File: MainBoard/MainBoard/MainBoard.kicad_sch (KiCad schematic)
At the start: 40 parts, among them IC1 BQ25171QWDRCRQ1, J1 KH-TYPE-C-16P, U1 STM32L496VGY6PTR, U2 MX25R1635FZUIL0, U3 SI3477DV-T1-GE3, U4 SI3477DV-T1-GE3, U5 TPS63802DLAR, U6 FUSB302BMPX

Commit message: Schematic work
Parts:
- added C21: 1uF, Capacitor_SMD:C_0402_1005Metric_Pad0.74x0.62mm_HandSolder, symbol Device:C
- added C22: 100nF, Capacitor_SMD:C_0402_1005Metric_Pad0.74x0.62mm_HandSolder, symbol Device:C
- added C23, C24: 470pF, Capacitor_SMD:C_0402_1005Metric_Pad0.74x0.62mm_HandSolder, symbol Device:C
- added R8, R9: 4.7k, Resistor_SMD:R_0402_1005Metric_Pad0.72x0.64mm_HandSolder, symbol Device:R_US
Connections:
- net +3.3V: now also C19.1, C20.1, R6.1, U5.6 (VOUT), U6.3 (VDD), U6.4 (VDD), C21.1, C22.1
- net GND: now also U6.15 (EPAD), U6.8 (GND), U6.9 (GND), C21.2, C22.2, C23.2, C24.2, R8.2, R9.1
- net at D1.2 (A), J1.A4_B9 (VBUS), J1.A9_B4 (VBUS): now also U6.2 (VBUS)
- net at J1.A5 (CC1): now also U6.11 (CC1), C24.1
- net at J1.B5 (CC2): now also U6.14 (CC2), C23.1
- net I2C1_SCL: now reaches U6.6 (SCL)
- net I2C1_SCL: now also R8.1
- net I2C1_SDA: now reaches U6.7 (SDA)
- net I2C1_SDA: now also R9.2
- no-connect marks 9 -> 12
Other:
- note added: "3.3V Regulator"
- note added: "Batteries"
- note added: "Battery Managment"
- note added: "Extra Flash"
- note added: "USBC + PD"
- moved on the sheet: BT1, BT2, C1, C10, C11, C12, C13, C14, C15, C16, C17, C18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

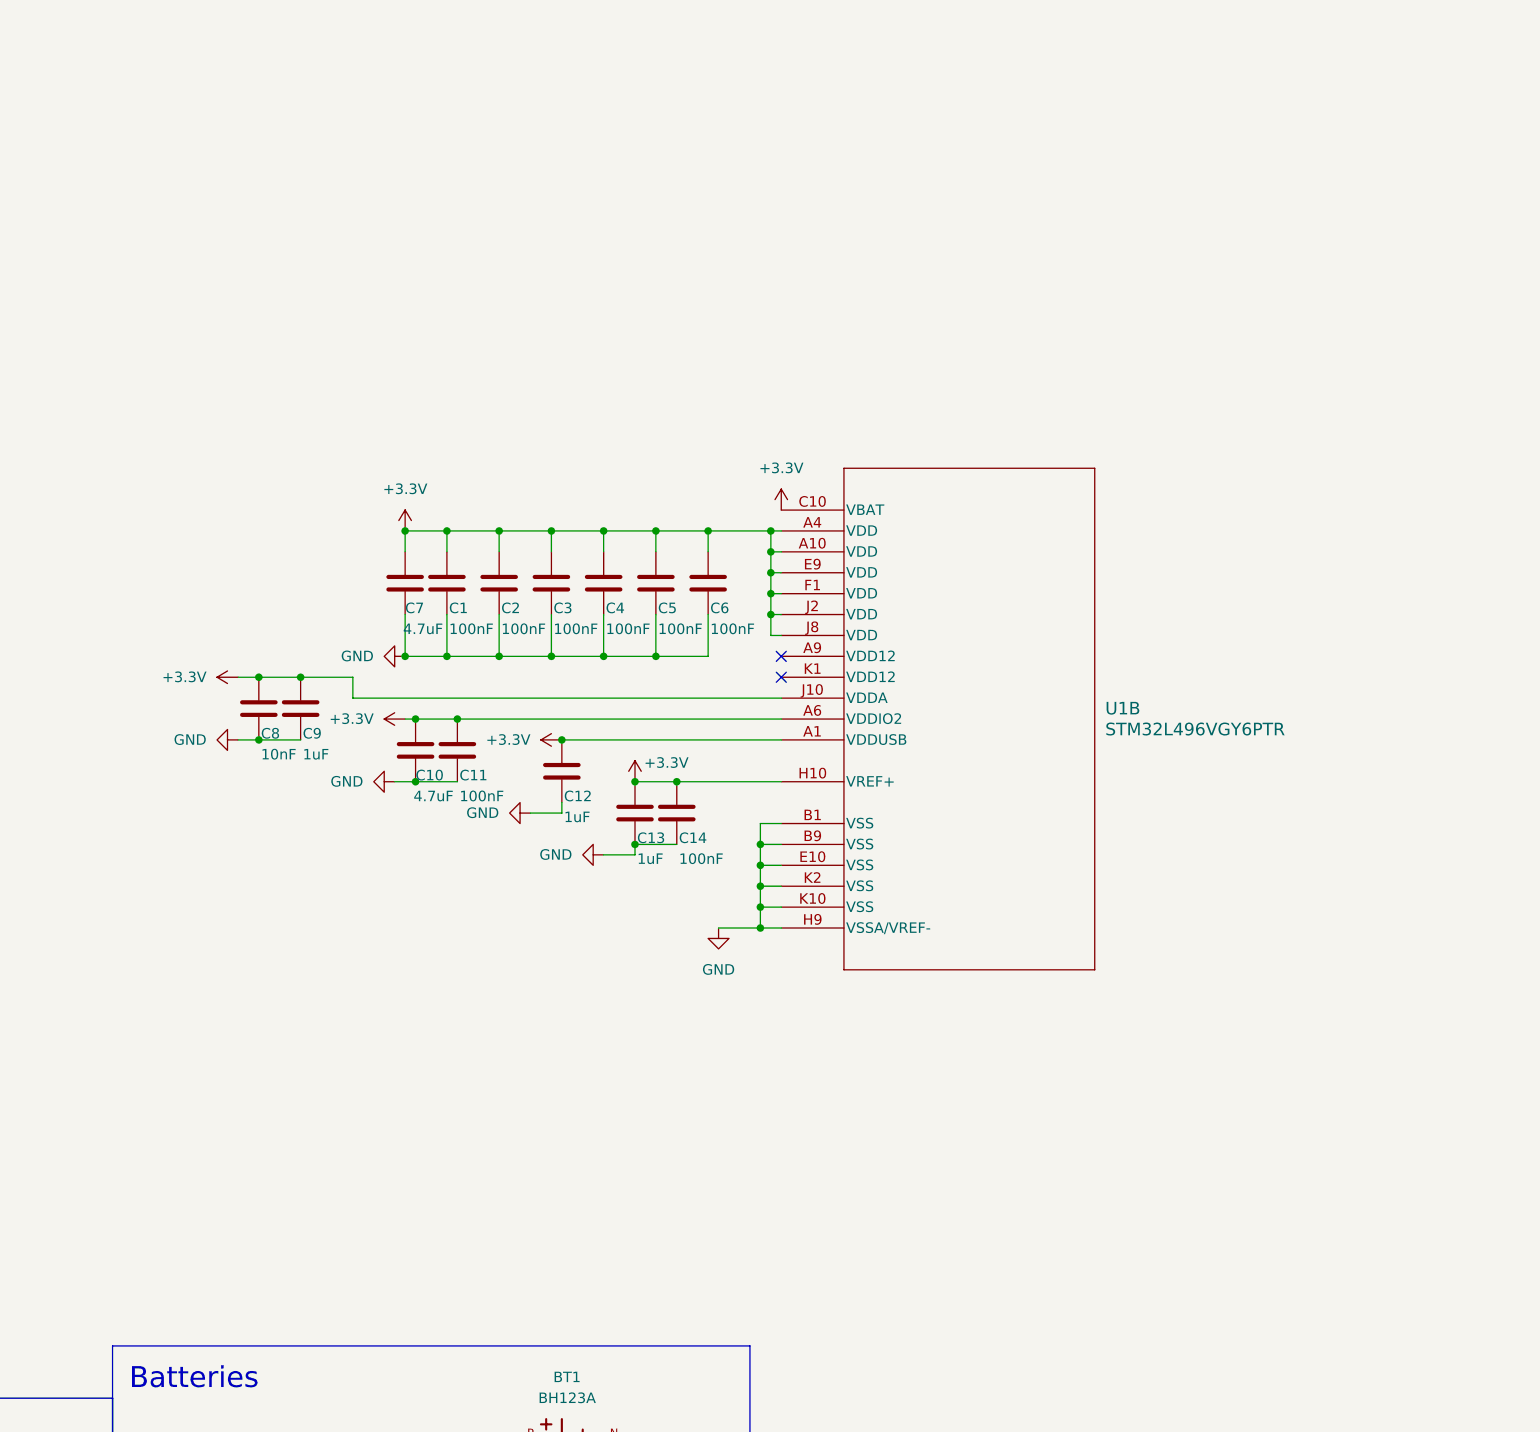
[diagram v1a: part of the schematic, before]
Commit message: Schematic Work
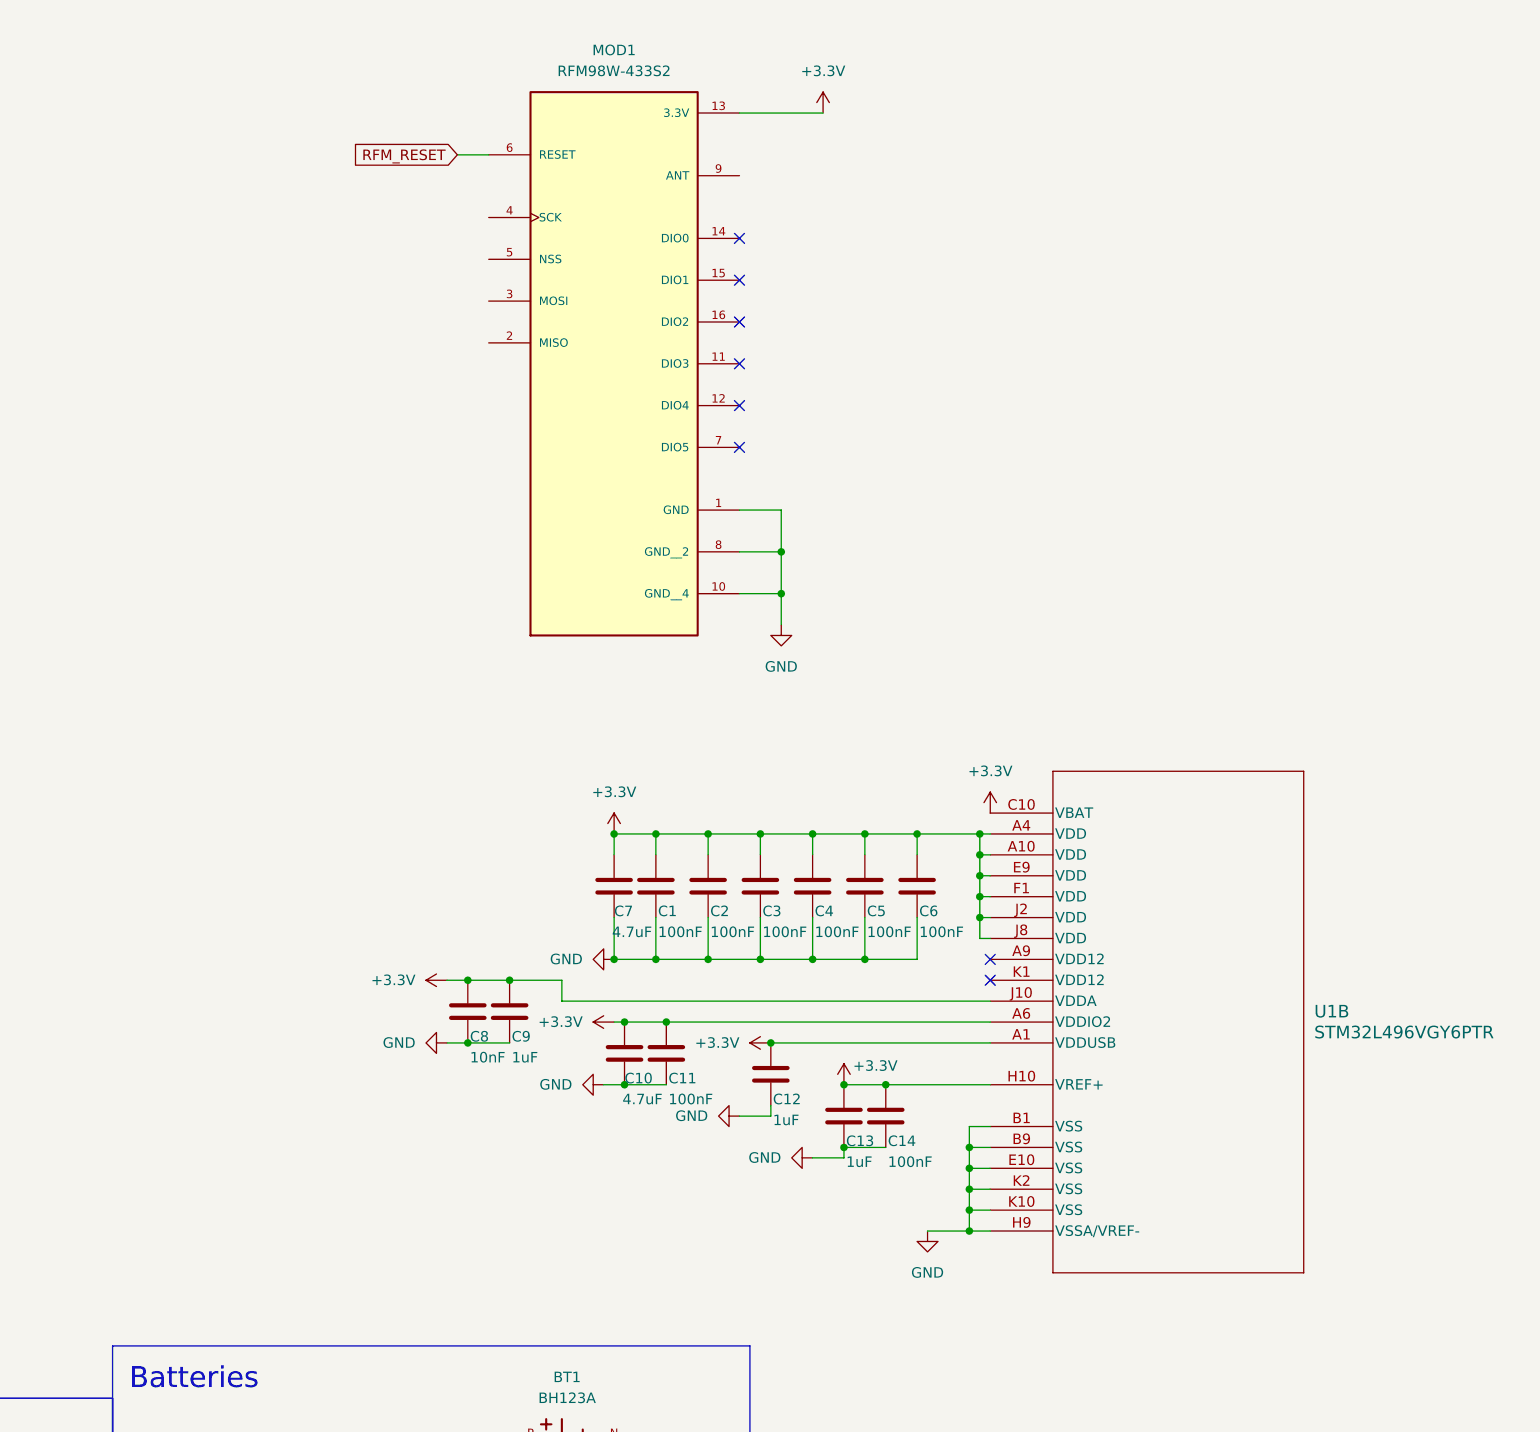
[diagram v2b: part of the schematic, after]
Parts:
- added MOD1: RFM98W-433S2, inspirefly:XCVR_RFM98W-433S2, symbol inspirefly:RFM98W-433S2
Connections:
- net +3.3V: now also MOD1.13 (3.3V)
- net GND: now also MOD1.1 (GND), MOD1.10 (GND__4), MOD1.8 (GND__2)
- new net RFM_RESET: MOD1.6 (RESET)
- no-connect marks 12 -> 18
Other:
- moved on the sheet: C1, C10, C11, C12, C13, C14, C2, C3, C4, C5, C6, C7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

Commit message: Schematic work
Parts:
- added C25, C26, C27: 100nF, Capacitor_SMD:C_0402_1005Metric_Pad0.74x0.62mm_HandSolder, symbol Device:C
- added C28, C29: 22pF, Capacitor_SMD:C_0402_1005Metric_Pad0.74x0.62mm_HandSolder, symbol Device:C
- added R10: 10k, Resistor_SMD:R_0402_1005Metric_Pad0.72x0.64mm_HandSolder, symbol Device:R_US
- added U7: BNO086, inspirefly:BNO086, symbol inspirefly:BNO086
- added Y1: 9HT11-32.768KBZF-T, Crystal:Crystal_SMD_2012-2Pin_2.0x1.2mm_HandSoldering, symbol Device:Crystal
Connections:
- net +3.3V: now also C25.2, C26.1, R10.1, U7.28 (VDDIO), U7.3 (VDD), U7.5 (PS1)
- net GND: now also C25.1, C26.2, C27.2, C28.2, C29.1, U7.2 (GND_1), U7.25 (GND_2)
- net CHARGE_DISABLE: now reaches IC1.3 (~{CE})
- new net: C29.2, U7.27 (XIN32), Y1.1
- new net: C28.1, U7.26 (XOUT32/CLKSEL1), Y1.2
- new net: C27.1, U7.9 (CAP)
- new net IMU_BOOTN: R10.2, U7.4 (BOOTN)
- no-connect marks 18 -> 28
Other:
- moved on the sheet: MOD1, R2, U4

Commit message: Sorting Schematic
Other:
- note added: "Battery Heater Connection"
- note added: "Board Connector System - Using Harwin M55 Series"
- note added: "IMU"
- note added: "Microcontroller Power"
- note added: "Microcontroller Signals"
- note added: "Radio Module"
- moved on the sheet: BT1, BT2, C1, C10, C11, C12, C13, C14, C15, C16, C17, C18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
